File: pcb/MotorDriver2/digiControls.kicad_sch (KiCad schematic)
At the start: 22 parts, among them IC2 CP2102N-A02-GQFN20R, J1 USB4110-GF-A, U1 NCP361SNT1G, U2 MAX40200AUK, U3 XIAO-ESP32-C5-DIP, U7 USBLC6-2SC6

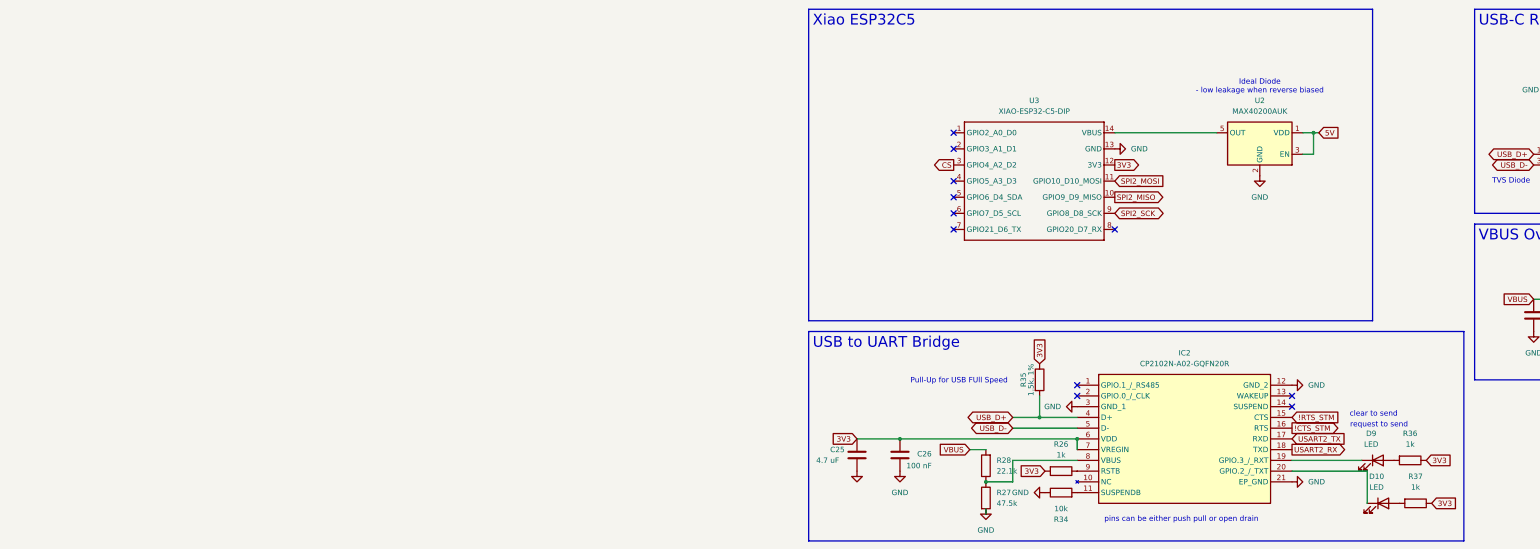
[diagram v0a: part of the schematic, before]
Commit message: Added step files
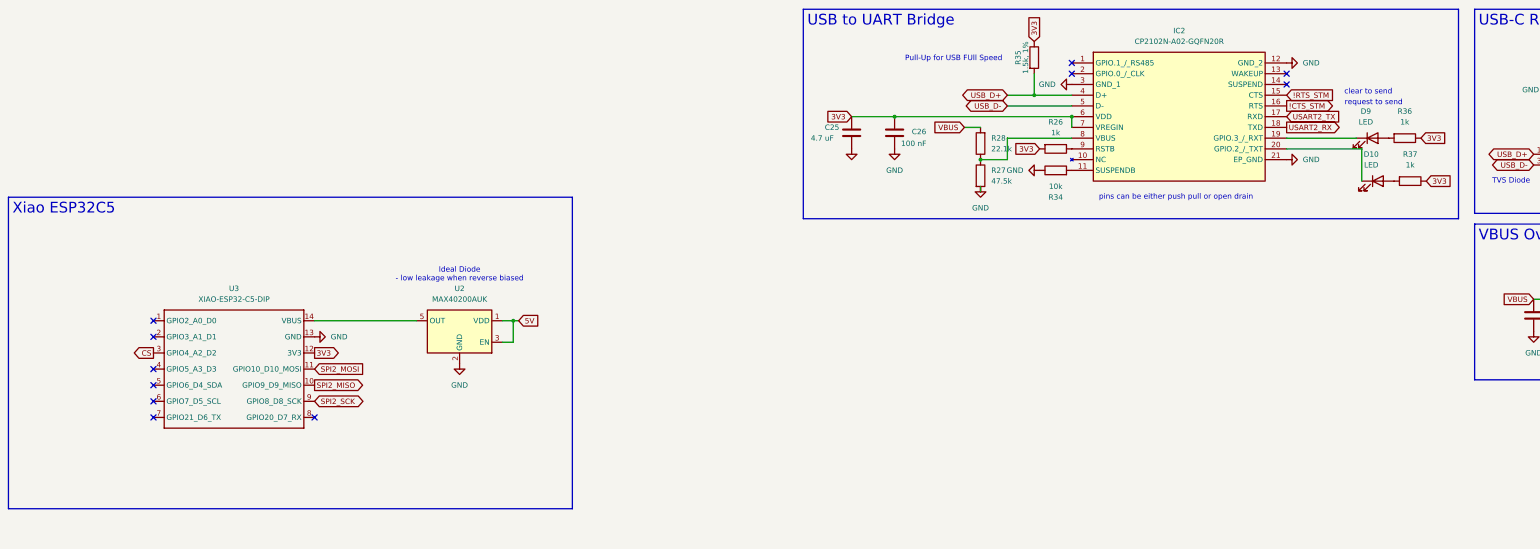
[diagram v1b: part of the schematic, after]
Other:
- moved on the sheet: C25, C26, D10, D9, IC2, R26, R27, R28, R34, R35, R36, R37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
